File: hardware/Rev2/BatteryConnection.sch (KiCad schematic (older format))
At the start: 3 parts

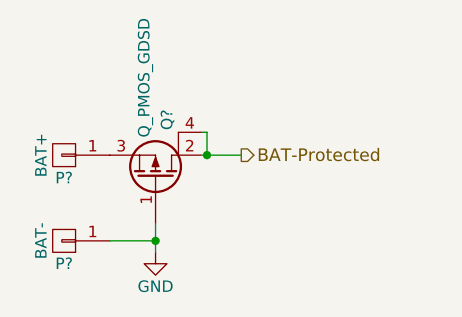
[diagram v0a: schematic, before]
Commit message: created PCB and gerbers
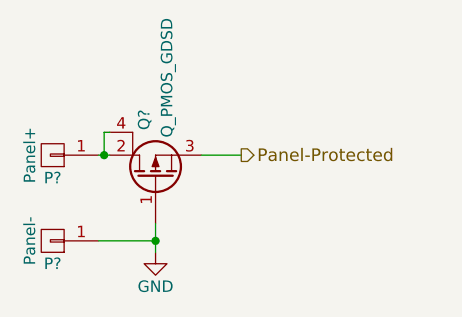
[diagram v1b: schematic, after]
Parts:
- P?: value BAT+ -> Panel+
- P?: value BAT- -> Panel-
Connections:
- net BAT-Protected is gone; now on an unnamed net: Q?.2 (D), Q?.4 (D)
- net at P?.1 (P1): no longer Q?.3 (S)
- new net Panel-Protected: Q?.3 (S)
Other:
- moved on the sheet: P?
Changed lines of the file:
@@
 LIBS:contrib
 LIBS:valves
+LIBS:PWM10-cache
 EELAYER 25 0
 EELAYER END
@@
 $EndDescr
 $Comp
-L Q_PMOS_GDSD Q?
-U 1 1 59250083
-P 4075 2875
-F 0 "Q?" H 4375 2925 50  0000 R CNN
-F 1 "Q_PMOS_GDSD" H 4775 2825 50  0000 R CNN
-F 2 "" H 4275 2975 50  0000 C CNN
-F 3 "" H 4075 2875 50  0000 C CNN
-	1    4075 2875
-	0    1    -1   0
-$EndComp
-$Comp
 L CONN_01X01 P?
 U 1 1 5925008A
-P 3675 2775
-F 0 "P?" H 3675 2875 50  0000 C CNN
-F 1 "BAT+" V 3775 2775 50  0000 C CNN
-F 2 "" H 3675 2775 50  0000 C CNN
-F 3 "" H 3675 2775 50  0000 C CNN
-	1    3675 2775
+P 3625 2775
+F 0 "P?" H 3625 2875 50  0000 C CNN
+F 1 "Panel+" V 3725 2775 50  0000 C CNN
+F 2 "" H 3625 2775 50  0000 C CNN
+F 3 "" H 3625 2775 50  0000 C CNN
+	1    3625 2775
 	-1   0    0    1
 $EndComp
@@
 L CONN_01X01 P?
 U 1 1 59250091
-P 3675 3150
-F 0 "P?" H 3675 3250 50  0000 C CNN
-F 1 "BAT-" V 3775 3150 50  0000 C CNN
-F 2 "" H 3675 3150 50  0000 C CNN
-F 3 "" H 3675 3150 50  0000 C CNN
-	1    3675 3150
+P 3625 3150
+F 0 "P?" H 3625 3250 50  0000 C CNN
+F 1 "Panel-" V 3725 3150 50  0000 C CNN
+F 2 "" H 3625 3150 50  0000 C CNN
+F 3 "" H 3625 3150 50  0000 C CNN
+	1    3625 3150
 	-1   0    0    1
 $EndComp
 Wire Wire Line
-	4075 3075 4075 3150
+	4075 3075 4075 3200
 Wire Wire Line
-	4075 3150 4075 3200
+	4075 3150 3825 3150
 Wire Wire Line
-	4075 3150 3875 3150
-Wire Wire Line
-	4275 2675 4300 2675
-Wire Wire Line
-	4300 2675 4300 2775
-Wire Wire Line
-	4275 2775 4300 2775
-Wire Wire Line
-	4300 2775 4450 2775
-Connection ~ 4300 2775
+	4275 2775 4450 2775
 $Comp
 L GND #PWR?
@@
 Connection ~ 4075 3150
 Text HLabel 4450 2775 2    55   Output ~ 0
-BAT-Protected
+Panel-Protected
+$Comp
+L Q_PMOS_GDSD Q?
+U 1 1 59250083
+P 4075 2875
+F 0 "Q?" H 4375 2925 50  0000 R CNN
+F 1 "Q_PMOS_GDSD" H 4775 2825 50  0000 R CNN
+F 2 "" H 4275 2975 50  0000 C CNN
+F 3 "" H 4075 2875 50  0000 C CNN
+	1    4075 2875
+	0    -1   -1   0
+$EndComp
+Wire Wire Line
+	3825 2775 3875 2775
+Wire Wire Line
+	3875 2675 3850 2675
+Wire Wire Line
+	3850 2675 3850 2775
+Connection ~ 3850 2775
 $EndSCHEMATC
